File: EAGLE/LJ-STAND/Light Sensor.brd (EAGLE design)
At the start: 119 x 119 mm, 122 parts

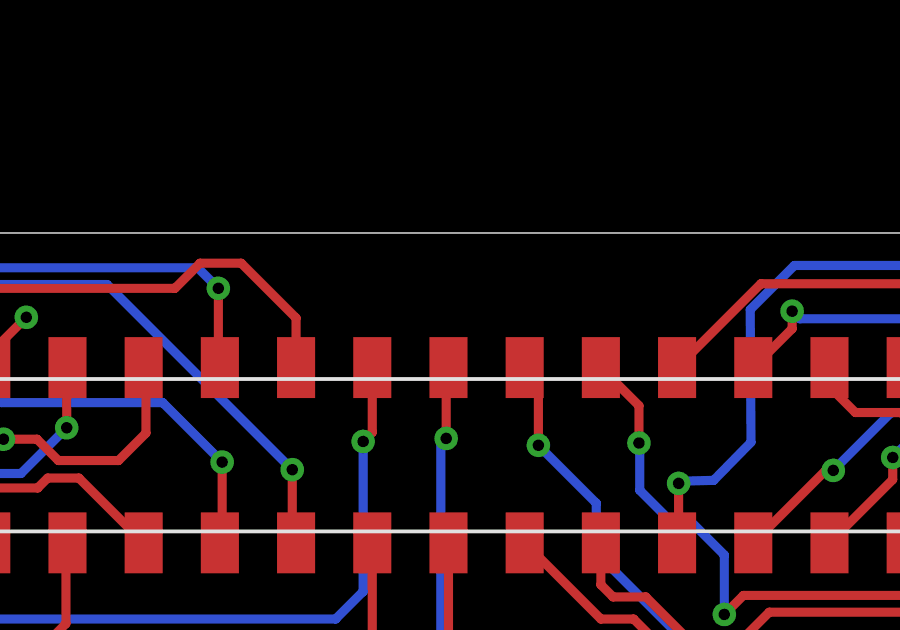
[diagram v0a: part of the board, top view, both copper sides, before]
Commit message: Main pcb
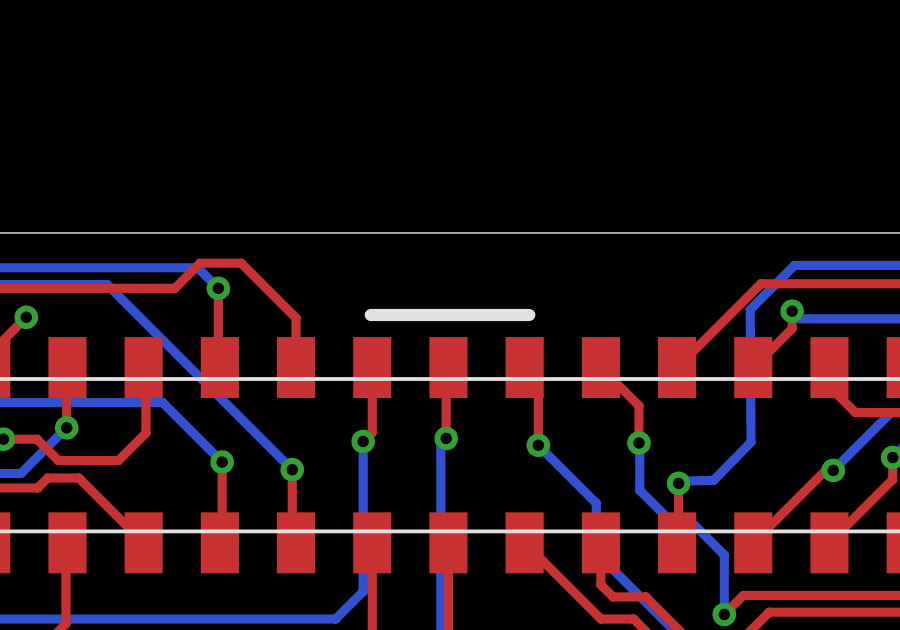
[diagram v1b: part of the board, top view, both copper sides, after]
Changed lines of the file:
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@@
 <rectangle x1="145.561053125" y1="149.44725" x2="149.767290625" y2="149.45486875" layer="21"/>
 <rectangle x1="145.568671875" y1="149.454871875" x2="149.759671875" y2="149.462490625" layer="21"/>
+<wire x1="146.2024" y1="69.5706" x2="151.4856" y2="69.5706" width="0.4064" layer="21"/>
 </plain>
 <attributes>
